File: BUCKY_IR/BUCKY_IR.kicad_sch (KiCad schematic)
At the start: 29 parts, among them J1 SERIAL_CONN, J2 CAN_CONN_UP, J3 CAN_CONN_DOWN, U1 TSSP96038TR, U10 TSSP96038TR, U11 TSSP96038TR, U12 TSSP96038TR, U13 TSSP96038TR, U14 TSSP96038TR, U15 TSSP96038TR, U16 TSSP96038TR, U17 SN65HVD230, U18 ESP32-WROOM-32D, U19 AMS1117, U2 TSSP96038TR, U3 TSSP96038TR, U4 TSSP96038TR, U5 TSSP96038TR, U6 TSSP96038TR, U7 TSSP96038TR, U8 TSSP96038TR, U9 TSSP96038TR

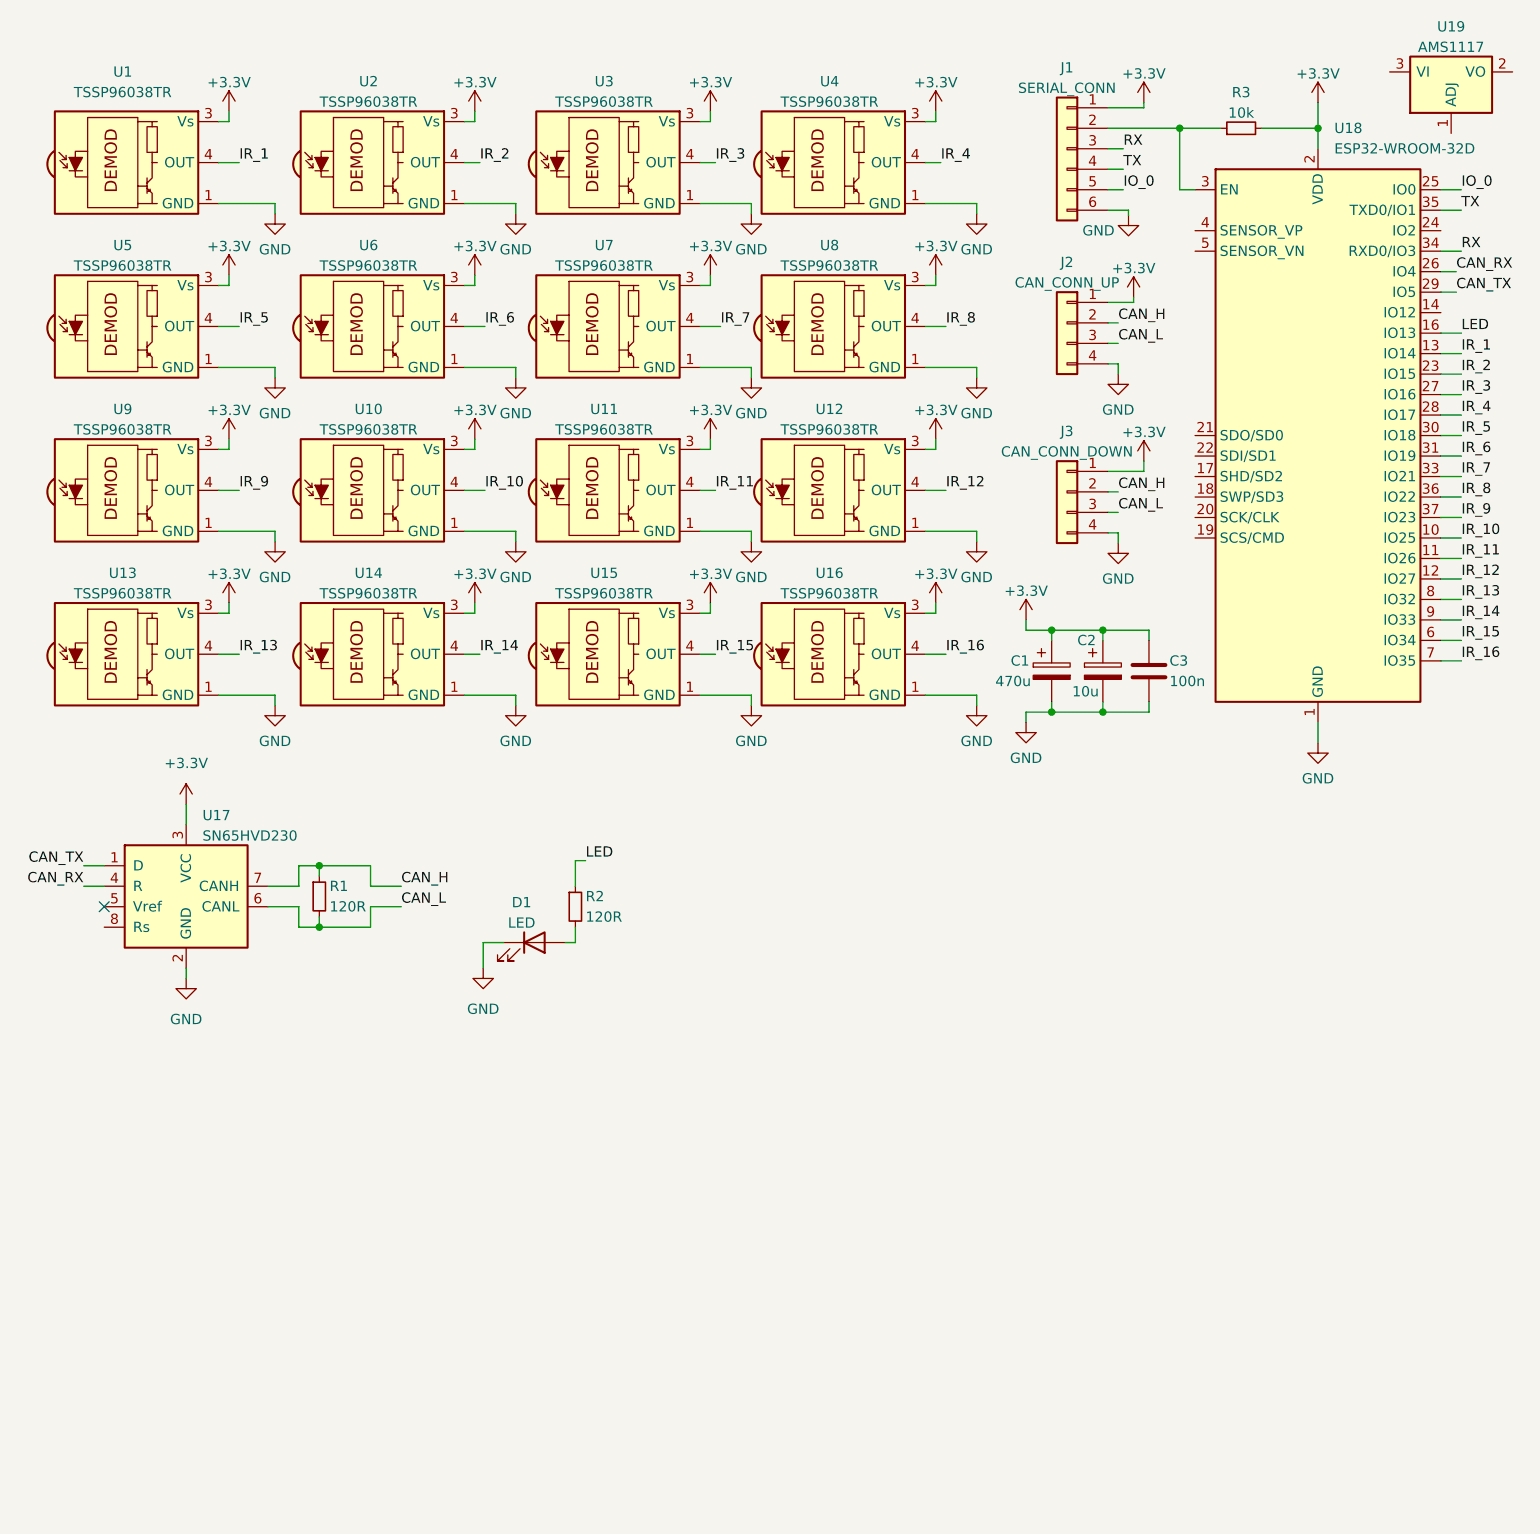
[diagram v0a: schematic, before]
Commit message: More IR dev
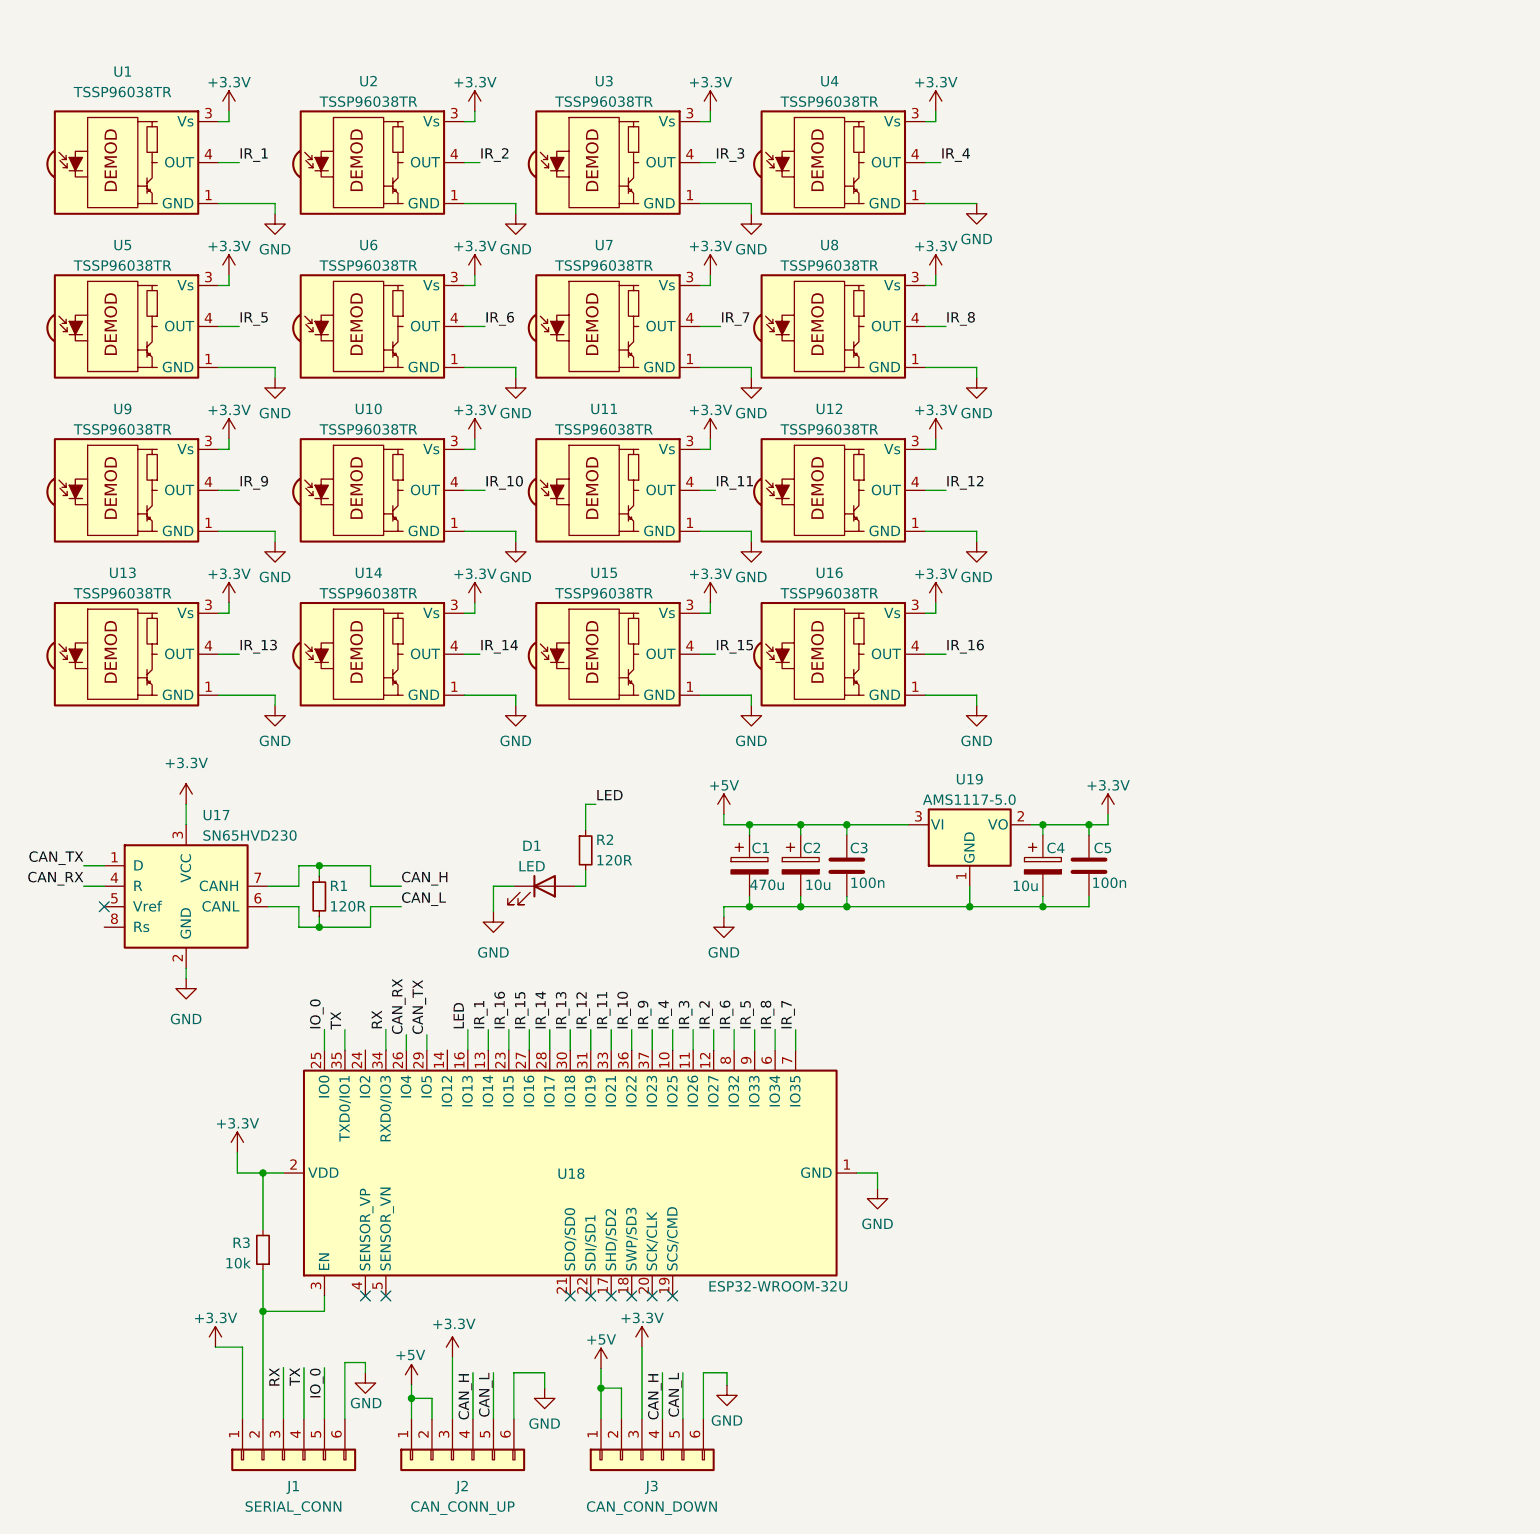
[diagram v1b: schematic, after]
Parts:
- removed J2: CAN_CONN_UP, Connector_JST:JST_PH_B6B-PH-K_1x06_P2.00mm_Vertical, symbol Connector_Generic:Conn_01x04
- removed J3: CAN_CONN_DOWN, Connector_JST:JST_PH_B6B-PH-K_1x06_P2.00mm_Vertical, symbol Connector_Generic:Conn_01x04
- removed U19: AMS1117, Package_TO_SOT_SMD:SOT-223-3_TabPin2, symbol Regulator_Linear:AMS1117
- added C4: 10u, Capacitor_SMD:CP_Elec_6.3x7.7, symbol Device:C_Polarized
- added C5: 100n, Capacitor_SMD:C_0805_2012Metric_Pad1.18x1.45mm_HandSolder, symbol Device:C
- added J2: CAN_CONN_UP, Connector_JST:JST_PH_S6B-PH-SM4-TB_1x06-1MP_P2.00mm_Horizontal, symbol Connector_Generic:Conn_01x06
- added J3: CAN_CONN_DOWN, Connector_JST:JST_PH_S6B-PH-SM4-TB_1x06-1MP_P2.00mm_Horizontal, symbol Connector_Generic:Conn_01x06
- added U19: AMS1117-5.0, Package_TO_SOT_SMD:SOT-223-3_TabPin2, symbol Regulator_Linear:AMS1117-5.0
- J1: footprint Connector_JST:JST_PH_B6B-PH-K_1x06_P2.00mm_Vertical -> Connector_JST:JST_PH_S6B-PH-SM4-TB_1x06-1MP_P2.00mm_Horizontal
- U18: value ESP32-WROOM-32D -> ESP32-WROOM-32U; footprint RF_Module:ESP32-WROOM-32 -> RF_Module:ESP32-WROOM-32U; symbol RF_Module:ESP32-WROOM-32D -> RF_Module:ESP32-WROOM-32U
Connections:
- net +3V3: now also C4.1, C5.1, J2.3 (Pin_3), J3.3 (Pin_3), U19.2 (VO); no longer C1.1, C2.1, C3.1
- net CAN_H: now also J2.4 (Pin_4), J3.4 (Pin_4)
- net CAN_L: now also J2.5 (Pin_5), J3.5 (Pin_5)
- net GND: now also C4.2, C5.2, J2.6 (Pin_6), J3.6 (Pin_6), U19.1 (GND)
- net IR_10: now also U18.36 (IO22); no longer U18.10 (IO25)
- net IR_11: now also U18.33 (IO21); no longer U18.11 (IO26)
- net IR_12: now also U18.31 (IO19); no longer U18.12 (IO27)
- net IR_13: now also U18.30 (IO18); no longer U18.8 (IO32)
- net IR_14: now also U18.28 (IO17); no longer U18.9 (IO33)
- net IR_15: now also U18.27 (IO16); no longer U18.6 (IO34)
- net IR_16: now also U18.23 (IO15); no longer U18.7 (IO35)
- net IR_2: now also U18.12 (IO27); no longer U18.23 (IO15)
- net IR_3: now also U18.11 (IO26); no longer U18.27 (IO16)
- net IR_4: now also U18.10 (IO25); no longer U18.28 (IO17)
- net IR_5: now also U18.9 (IO33); no longer U18.30 (IO18)
- net IR_6: now also U18.8 (IO32); no longer U18.31 (IO19)
- net IR_7: now also U18.7 (IO35); no longer U18.33 (IO21)
- net IR_8: now also U18.6 (IO34); no longer U18.36 (IO22)
- new net +5V: C1.1, C2.1, C3.1, J2.1 (Pin_1), J2.2 (Pin_2), J3.1 (Pin_1), J3.2 (Pin_2), U19.3 (VI)
- no-connect marks 1 -> 9
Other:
- moved on the sheet: C1, C2, C3, D1, J1, R2, R3, U18
